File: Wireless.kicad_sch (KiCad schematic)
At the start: 34 parts, among them J11 Conn_01x02_Pin, J16 Conn_01x04_Pin, J17 Conn_01x04_Pin, SW6 SW_Push, SW7 SW_Push, U14 ESP32-C3FH4, Y2 40MHz

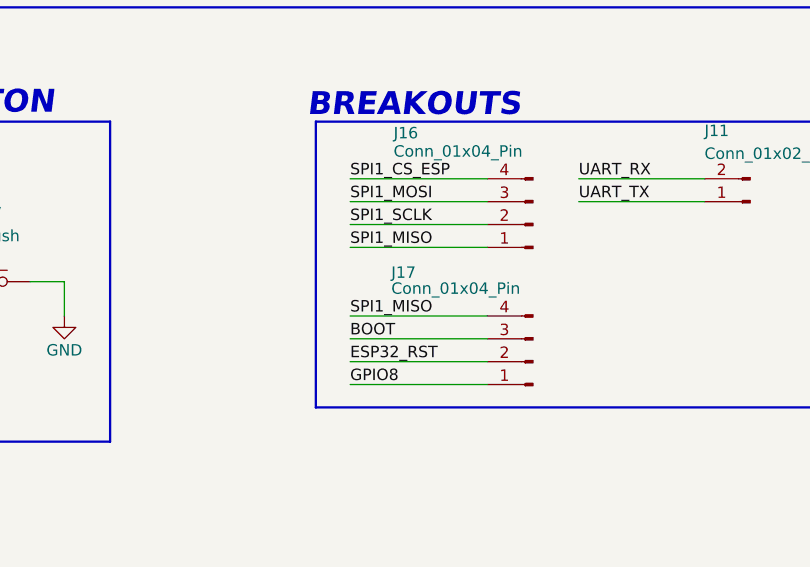
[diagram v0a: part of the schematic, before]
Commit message: saving to not lose prorgress
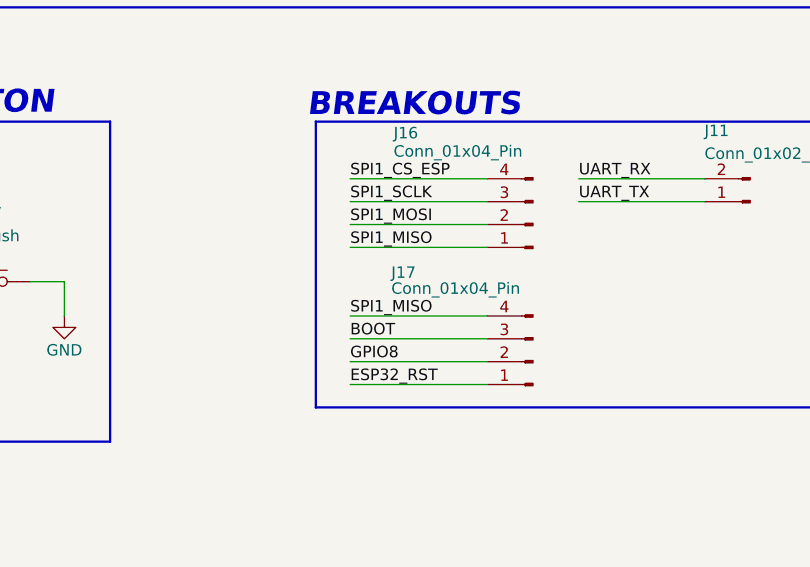
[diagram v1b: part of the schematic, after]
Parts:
- C28, C29: footprint Capacitor_SMD:C_0402_1005Metric_Pad0.74x0.62mm_HandSolder -> Capacitor_SMD:C_0201_0603Metric_Pad0.64x0.40mm_HandSolder
- L2: footprint Inductor_SMD:L_0402_1005Metric_Pad0.77x0.64mm_HandSolder -> Inductor_SMD:L_0201_0603Metric_Pad0.64x0.40mm_HandSolder
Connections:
- net ESP32_RST: now also J17.1 (Pin_1); no longer J17.2 (Pin_2)
- net GPIO8: now also J17.2 (Pin_2); no longer J17.1 (Pin_1)
- net SPI1_MOSI: now also J16.2 (Pin_2); no longer J16.3 (Pin_3)
- net SPI1_SCLK: now also J16.3 (Pin_3); no longer J16.2 (Pin_2)
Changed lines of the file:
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@@
 	(wire
 		(pts
-			(xy 190.5 135.89) (xy 205.74 135.89)
+			(xy 171.45 38.1) (xy 173.99 38.1)
 		)
 		(stroke
@@
 	(wire
 		(pts
-			(xy 171.45 38.1) (xy 173.99 38.1)
+			(xy 52.07 175.26) (xy 52.07 176.53)
 		)
 		(stroke
@@
 	(wire
 		(pts
-			(xy 52.07 175.26) (xy 52.07 176.53)
+			(xy 190.5 153.67) (xy 205.74 153.67)
 		)
 		(stroke
@@
 	(wire
 		(pts
-			(xy 190.5 156.21) (xy 205.74 156.21)
+			(xy 41.91 88.9) (xy 41.91 92.71)
 		)
 		(stroke
@@
 	(wire
 		(pts
-			(xy 41.91 88.9) (xy 41.91 92.71)
+			(xy 190.5 138.43) (xy 205.74 138.43)
 		)
 		(stroke
@@
 	(wire
 		(pts
-			(xy 166.37 35.56) (xy 166.37 41.91)
+			(xy 190.5 135.89) (xy 205.74 135.89)
 		)
 		(stroke
@@
 	(wire
 		(pts
-			(xy 34.29 165.1) (xy 52.07 165.1)
+			(xy 166.37 35.56) (xy 166.37 41.91)
 		)
 		(stroke
@@
 	(wire
 		(pts
-			(xy 190.5 153.67) (xy 205.74 153.67)
+			(xy 34.29 165.1) (xy 52.07 165.1)
 		)
 		(stroke
@@
 	(wire
 		(pts
-			(xy 57.15 38.1) (xy 59.69 38.1)
+			(xy 190.5 156.21) (xy 205.74 156.21)
 		)
 		(stroke
@@
 	(wire
 		(pts
-			(xy 22.86 151.13) (xy 52.07 151.13)
+			(xy 57.15 38.1) (xy 59.69 38.1)
 		)
 		(stroke
@@
 	(wire
 		(pts
-			(xy 215.9 135.89) (xy 229.87 135.89)
+			(xy 22.86 151.13) (xy 52.07 151.13)
 		)
 		(stroke
@@
 	(wire
 		(pts
-			(xy 158.75 144.78) (xy 154.94 144.78)
+			(xy 215.9 135.89) (xy 229.87 135.89)
 		)
 		(stroke
@@
 	(wire
 		(pts
-			(xy 21.59 175.26) (xy 52.07 175.26)
+			(xy 158.75 144.78) (xy 154.94 144.78)
 		)
 		(stroke
@@
 	(wire
 		(pts
-			(xy 22.86 149.86) (xy 22.86 151.13)
+			(xy 21.59 175.26) (xy 52.07 175.26)
 		)
 		(stroke
@@
 	(wire
 		(pts
-			(xy 207.01 54.61) (xy 227.33 54.61)
+			(xy 22.86 149.86) (xy 22.86 151.13)
 		)
 		(stroke
@@
 	(wire
 		(pts
-			(xy 190.5 138.43) (xy 205.74 138.43)
+			(xy 207.01 54.61) (xy 227.33 54.61)
 		)
 		(stroke
@@
 	)
 	(label "SPI1_MOSI"
-		(at 190.5 135.89 0)
+		(at 190.5 138.43 0)
 		(effects
 			(font
@@
 	)
 	(label "SPI1_SCLK"
-		(at 190.5 138.43 0)
+		(at 190.5 135.89 0)
 		(effects
 			(font
@@
 	)
 	(label "GPIO8"
-		(at 190.5 156.21 0)
+		(at 190.5 153.67 0)
 		(effects
 			(font
@@
 	)
 	(label "ESP32_RST"
-		(at 190.5 153.67 0)
+		(at 190.5 156.21 0)
 		(effects
 			(font
@@
 			)
 		)
-		(property "Footprint" "Inductor_SMD:L_0402_1005Metric_Pad0.77x0.64mm_HandSolder"
+		(property "Footprint" "Inductor_SMD:L_0201_0603Metric_Pad0.64x0.40mm_HandSolder"
 			(at 53.34 38.1 0)
 			(hide yes)
@@
 			)
 		)
-		(property "Footprint" "Capacitor_SMD:C_0402_1005Metric_Pad0.74x0.62mm_HandSolder"
+		(property "Footprint" "Capacitor_SMD:C_0201_0603Metric_Pad0.64x0.40mm_HandSolder"
 			(at 60.6552 48.26 0)
 			(hide yes)
@@
 			)
 		)
-		(property "Footprint" "Capacitor_SMD:C_0402_1005Metric_Pad0.74x0.62mm_HandSolder"
+		(property "Footprint" "Capacitor_SMD:C_0201_0603Metric_Pad0.64x0.40mm_HandSolder"
 			(at 47.9552 48.26 0)
 			(hide yes)

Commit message: ESP32 Routing
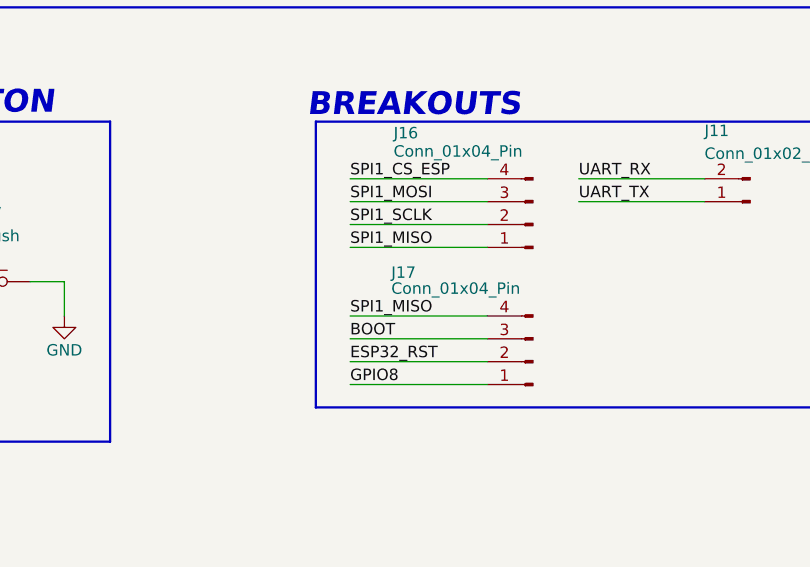
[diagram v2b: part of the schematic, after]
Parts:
- C28, C29: footprint Capacitor_SMD:C_0201_0603Metric_Pad0.64x0.40mm_HandSolder -> Capacitor_SMD:C_0402_1005Metric_Pad0.74x0.62mm_HandSolder
- L2: footprint Inductor_SMD:L_0201_0603Metric_Pad0.64x0.40mm_HandSolder -> Inductor_SMD:L_0402_1005Metric_Pad0.77x0.64mm_HandSolder
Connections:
- net ESP32_RST: now also J17.2 (Pin_2); no longer J17.1 (Pin_1)
- net GPIO8: now also J17.1 (Pin_1); no longer J17.2 (Pin_2)
- net SPI1_MOSI: now also J16.3 (Pin_3); no longer J16.2 (Pin_2)
- net SPI1_SCLK: now also J16.2 (Pin_2); no longer J16.3 (Pin_3)
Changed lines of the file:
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@@
 	(wire
 		(pts
-			(xy 171.45 38.1) (xy 173.99 38.1)
+			(xy 190.5 135.89) (xy 205.74 135.89)
 		)
 		(stroke
@@
 	(wire
 		(pts
-			(xy 52.07 175.26) (xy 52.07 176.53)
+			(xy 171.45 38.1) (xy 173.99 38.1)
 		)
 		(stroke
@@
 	(wire
 		(pts
-			(xy 190.5 153.67) (xy 205.74 153.67)
+			(xy 52.07 175.26) (xy 52.07 176.53)
 		)
 		(stroke
@@
 	(wire
 		(pts
-			(xy 41.91 88.9) (xy 41.91 92.71)
+			(xy 190.5 156.21) (xy 205.74 156.21)
 		)
 		(stroke
@@
 	(wire
 		(pts
-			(xy 190.5 138.43) (xy 205.74 138.43)
+			(xy 41.91 88.9) (xy 41.91 92.71)
 		)
 		(stroke
@@
 	(wire
 		(pts
-			(xy 190.5 135.89) (xy 205.74 135.89)
+			(xy 166.37 35.56) (xy 166.37 41.91)
 		)
 		(stroke
@@
 	(wire
 		(pts
-			(xy 166.37 35.56) (xy 166.37 41.91)
+			(xy 34.29 165.1) (xy 52.07 165.1)
 		)
 		(stroke
@@
 	(wire
 		(pts
-			(xy 34.29 165.1) (xy 52.07 165.1)
+			(xy 190.5 153.67) (xy 205.74 153.67)
 		)
 		(stroke
@@
 	(wire
 		(pts
-			(xy 190.5 156.21) (xy 205.74 156.21)
+			(xy 57.15 38.1) (xy 59.69 38.1)
 		)
 		(stroke
@@
 	(wire
 		(pts
-			(xy 57.15 38.1) (xy 59.69 38.1)
+			(xy 22.86 151.13) (xy 52.07 151.13)
 		)
 		(stroke
@@
 	(wire
 		(pts
-			(xy 22.86 151.13) (xy 52.07 151.13)
+			(xy 215.9 135.89) (xy 229.87 135.89)
 		)
 		(stroke
@@
 	(wire
 		(pts
-			(xy 215.9 135.89) (xy 229.87 135.89)
+			(xy 158.75 144.78) (xy 154.94 144.78)
 		)
 		(stroke
@@
 	(wire
 		(pts
-			(xy 158.75 144.78) (xy 154.94 144.78)
+			(xy 21.59 175.26) (xy 52.07 175.26)
 		)
 		(stroke
@@
 	(wire
 		(pts
-			(xy 21.59 175.26) (xy 52.07 175.26)
+			(xy 22.86 149.86) (xy 22.86 151.13)
 		)
 		(stroke
@@
 	(wire
 		(pts
-			(xy 22.86 149.86) (xy 22.86 151.13)
+			(xy 207.01 54.61) (xy 227.33 54.61)
 		)
 		(stroke
@@
 	(wire
 		(pts
-			(xy 207.01 54.61) (xy 227.33 54.61)
+			(xy 190.5 138.43) (xy 205.74 138.43)
 		)
 		(stroke
@@
 	)
 	(label "SPI1_MOSI"
-		(at 190.5 138.43 0)
+		(at 190.5 135.89 0)
 		(effects
 			(font
@@
 	)
 	(label "SPI1_SCLK"
-		(at 190.5 135.89 0)
+		(at 190.5 138.43 0)
 		(effects
 			(font
@@
 	)
 	(label "GPIO8"
-		(at 190.5 153.67 0)
+		(at 190.5 156.21 0)
 		(effects
 			(font
@@
 	)
 	(label "ESP32_RST"
-		(at 190.5 156.21 0)
+		(at 190.5 153.67 0)
 		(effects
 			(font
@@
 			)
 		)
-		(property "Footprint" "Inductor_SMD:L_0201_0603Metric_Pad0.64x0.40mm_HandSolder"
+		(property "Footprint" "Inductor_SMD:L_0402_1005Metric_Pad0.77x0.64mm_HandSolder"
 			(at 53.34 38.1 0)
 			(hide yes)
@@
 			)
 		)
-		(property "Footprint" "Capacitor_SMD:C_0201_0603Metric_Pad0.64x0.40mm_HandSolder"
+		(property "Footprint" "Capacitor_SMD:C_0402_1005Metric_Pad0.74x0.62mm_HandSolder"
 			(at 60.6552 48.26 0)
 			(hide yes)
@@
 			)
 		)
-		(property "Footprint" "Capacitor_SMD:C_0201_0603Metric_Pad0.64x0.40mm_HandSolder"
+		(property "Footprint" "Capacitor_SMD:C_0402_1005Metric_Pad0.74x0.62mm_HandSolder"
 			(at 47.9552 48.26 0)
 			(hide yes)
